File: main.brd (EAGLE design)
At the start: 24.4 x 26.2 mm, 38 parts, among them IC1 ATTINY13A-SSH, IC2 TP4056-42-ESOP8, IC3 LM27313XMFX_NOPB, IC4 TPL5110DDCT, T1A 2N4401, T1B NPN, X1 MINI-USB-UX60A-MB-5ST, X2 332-02

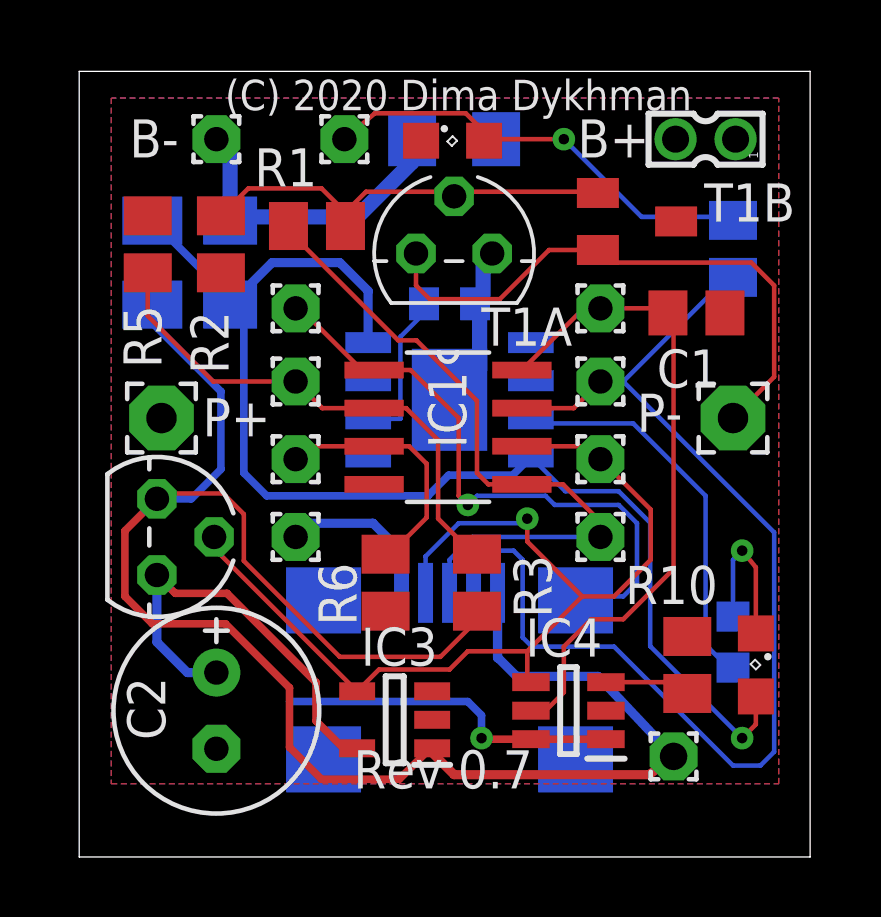
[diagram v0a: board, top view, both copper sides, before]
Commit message: many updates
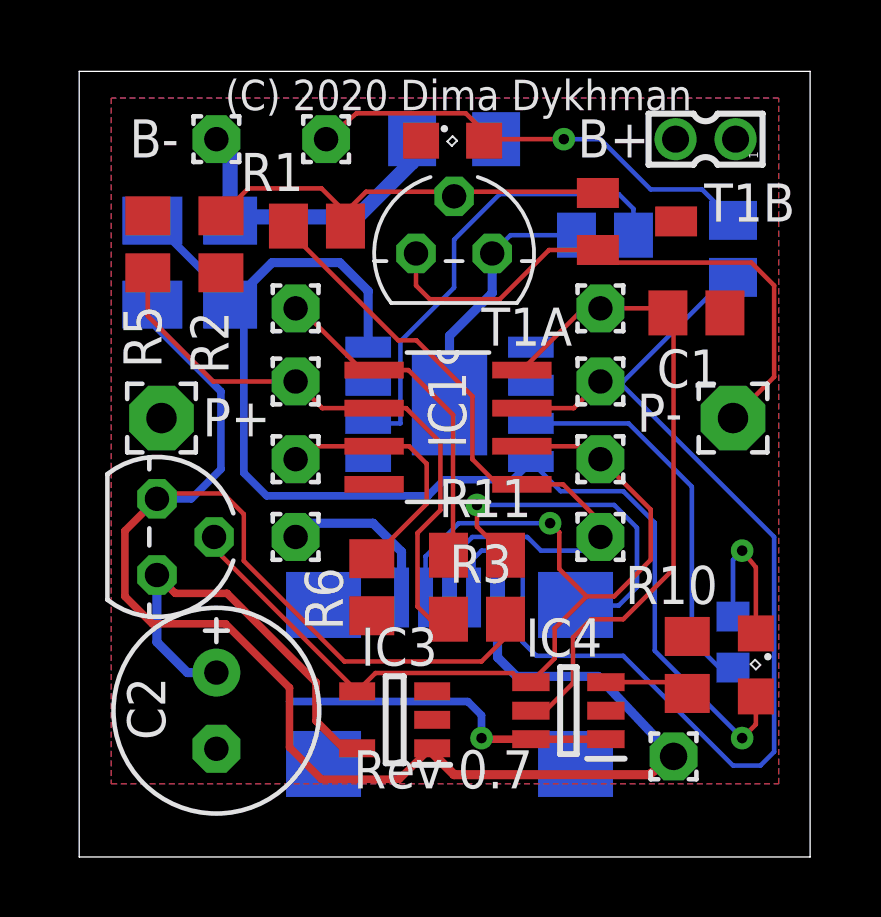
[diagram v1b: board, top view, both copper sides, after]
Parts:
- added R11: 10k, resistor:R0805
- R1: value 510 -> 1k; device resistor:M0805 -> resistor:R0805
- R10, R2, R5, R6: device resistor:M0805 -> resistor:R0805
- R3: value 10k -> 1k; device resistor:M0805 -> resistor:R0805
- R7: value 510 -> 1k
- R9: device rcl:R0603 -> rcl:R0805
- moved R9 5.66 mm to (18.4, 19.8), turned to 0 degrees
- moved R3 1.22 mm to (14.2, 7.01), turned to 0 degrees
- moved PAD1 0.61 mm to (9.14, 23.0)
- moved R6 0.48 mm to (10.7, 8.08)
- moved IC2 0.15 mm to (13.3, 14.2)
- moved X1 0.15 mm to (13.3, 5.49)
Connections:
- new net N$12: R11.2
- net RESET: now also R11.1
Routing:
- net N$12: track 0.00 -> 11.9 mm, vias 0 -> 1
- net N$11: track 5.24 -> 15.6 mm
- net RESET: track 19.9 -> 11.5 mm, vias 1 -> 0
- net GND: track 21.6 -> 24.9 mm
- net UART_TX: track 17.2 -> 19.9 mm
- net N$5: track 62.0 -> 60.9 mm
- net N$6: track 15.0 -> 15.6 mm

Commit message: updates
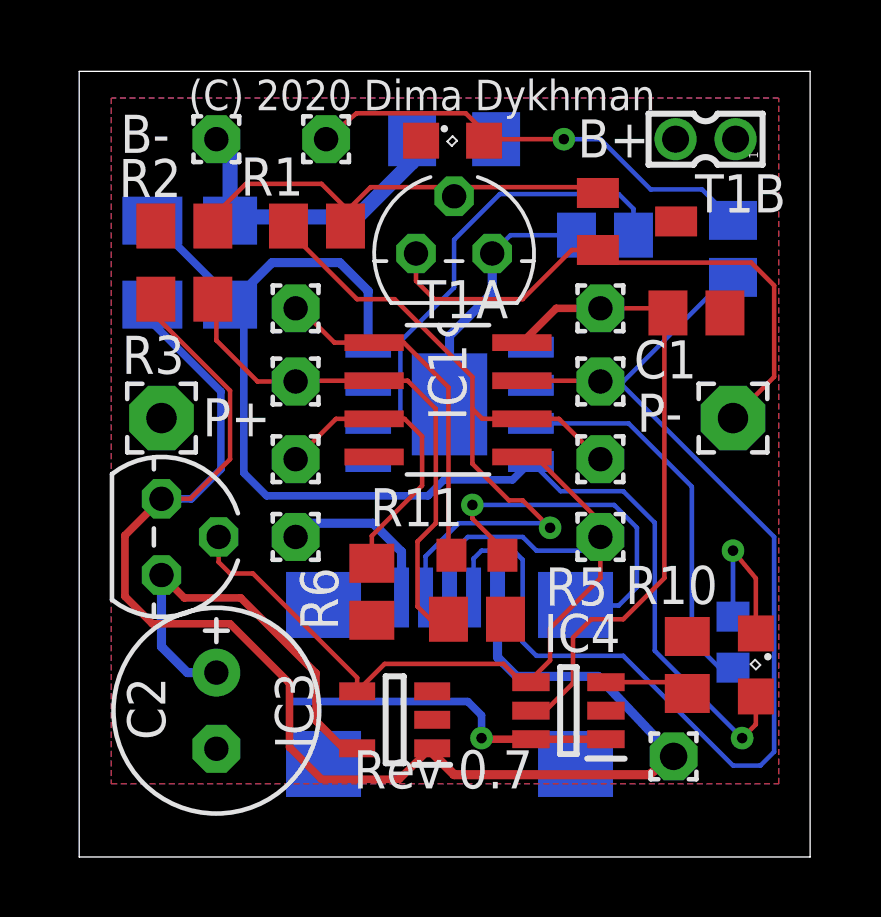
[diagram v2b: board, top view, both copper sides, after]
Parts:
- R11: device resistor:R0805 -> resistor:R0603
- R3: value 1k -> 330R
- R9: value 1.2k -> 2.2k
- moved R5 16.6 mm to (14.2, 7.01), turned to 0 degrees
- moved R3 14.5 mm to (4.42, 17.7), turned to 180 degrees
- moved R2 1.36 mm to (4.42, 20.1), turned to 0 degrees
- moved IC1 0.91 mm to (13.2, 14.3)
- moved REG1A 0.15 mm to (3.66, 9.75)
- moved R6 0.15 mm to (10.7, 7.92)
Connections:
- net UART_TX renamed SENSOR+
- removed net SENSOR/PUMP: IC1.5, PAD5.1, R1.2, X1.3
- removed net SOLAR: IC1.6, IC3.4, IC4.4, PAD6.1, REG1A.2, X1.4
- new net NPN+: IC1.6, PAD6.1, R1.2, X1.4
- new net SOLAR_REG+/-: IC1.5, IC3.4, IC4.4, PAD5.1, REG1A.2, X1.3
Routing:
- net SOLAR: track 35.3 -> 0.00 mm, vias 1 -> 0
- net SOLAR_REG+/-: track 0.00 -> 30.8 mm
- net NPN+: track 0.00 -> 25.7 mm, vias 0 -> 1
- net SENSOR/PUMP: track 23.3 -> 0.00 mm
- net N$5: track 60.9 -> 54.2 mm
- net SENSOR+: track 19.9 -> 17.8 mm
- net SENSOR-: track 8.71 -> 9.94 mm
- net N$1: track 14.2 -> 15.2 mm
- net N$3: track 22.0 -> 21.5 mm

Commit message: rev 0.8 (usbtiny built-in)
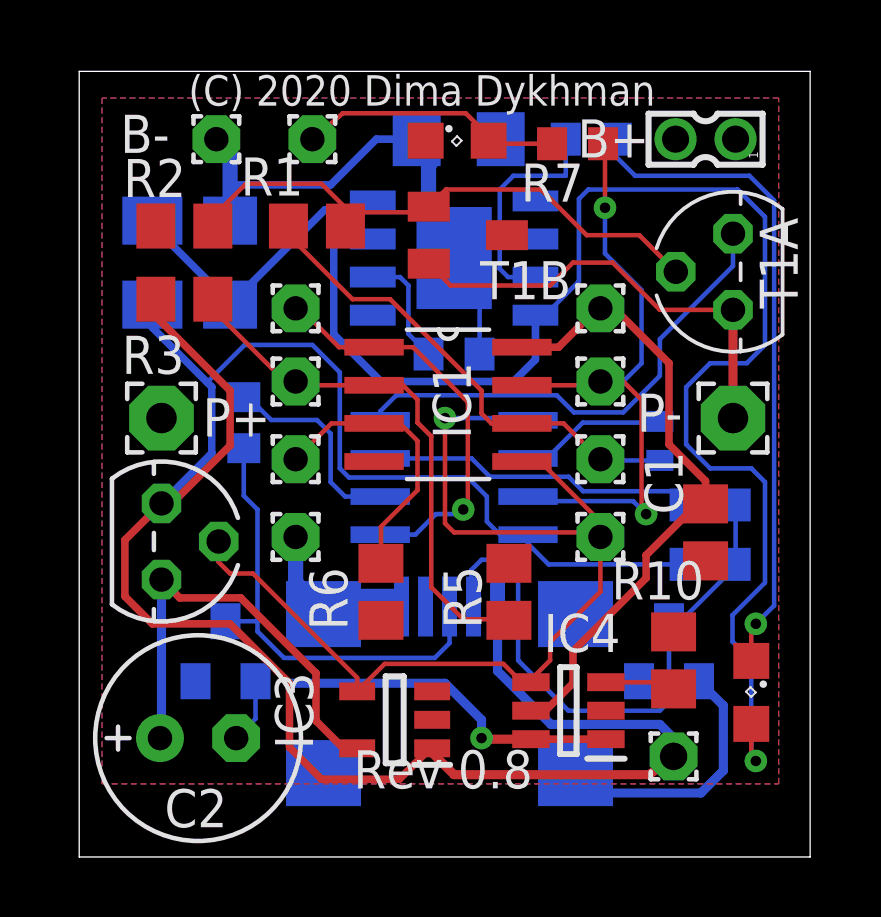
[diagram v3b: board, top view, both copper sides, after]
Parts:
- added D1, D2: BZX84CSMD, diode:TO236
- added IC5: ATTINY13A-SSH, STM32F103RBT6:SOIC127P600X175-8N
- added R12: 68R, resistor:R0603
- added R13: 1.5k, resistor:R0603
- added R14: 0R, resistor:R0402
- C4: device rcl:C3216 -> rcl:C1206
- R11: value 10k -> 68R
- R7: device resistor:M0805 -> resistor:R0603
- R9: device rcl:R0805 -> rcl:R0603
- moved R8 17.4 mm to (18.0, 23.0), turned to 0 degrees
- moved T1A 9.32 mm to (22.7, 18.6), turned to 90 degrees
- moved R11 7.95 mm to (21.9, 10.8), flipped to the bottom
- moved C1 7.32 mm to (21.8, 9.91), turned to 90 degrees
- moved R9 6.40 mm to (13.4, 15.8), turned to 180 degrees
- moved R7 6.26 mm to (17.5, 22.9), flipped to the top, turned to 180 degrees
- moved T1B 5.66 mm to (13.9, 19.8)
- moved IC2 4.88 mm to (13.4, 19.1)
- moved R5 1.41 mm to (15.2, 7.92), turned to 90 degrees
- moved C2 1.10 mm to (4.88, 3.05), turned to 0 degrees
- moved LED2 0.93 mm to (23.3, 4.57)
- moved R10 0.48 mm to (20.7, 5.64)
- moved PAD1 0.46 mm to (8.69, 23.0)
- moved R6 0.30 mm to (11.0, 7.92)
- moved X1 0.30 mm to (13.3, 5.18)
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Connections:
- new net N$10: IC5.3, R11.2
- new net N$13: D1.C, R11.1, R13.2, X1.2
- new net N$14: D2.C, R12.1, X1.3
- new net N$15: IC5.6, R14.1
- net GND: now also D1.A, D2.A, IC5.4
- net LED: now also IC5.7; no longer X1.2
- net N$12: now also IC5.2, R12.2; no longer R11.2
- net N$5: now also IC5.8, R13.1
- net NPN+: now also R14.2; no longer X1.4
- net RESET: now also IC5.1; no longer R11.1
- net SOLAR_REG+/-: now also IC5.5; no longer X1.3
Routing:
- net GND: track 24.9 -> 53.1 mm
- net N$5: track 54.2 -> 75.4 mm
- net N$13: track 0.00 -> 19.7 mm
- net LED: track 39.2 -> 21.8 mm, vias 0 -> 2
- net N$9: track 5.23 -> 22.1 mm
- net N$4: track 42.4 -> 58.6 mm
- net N$14: track 0.00 -> 15.6 mm
- net N$11: track 15.6 -> 3.87 mm
- net N$10: track 0.00 -> 10.8 mm
- net NPN+: track 25.7 -> 16.2 mm, vias 1 -> 0
- net N$6: track 15.6 -> 8.82 mm, vias 1 -> 0
- net N$8: track 13.1 -> 7.56 mm
- net N$12: track 12.1 -> 6.86 mm, vias 1 -> 0
- net N$15: track 0.00 -> 4.91 mm
- net SOLAR_REG+/-: track 30.8 -> 35.1 mm, vias 0 -> 1
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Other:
- board text added: "Rev 0.8"
- board text removed: "Rev 0.7"
